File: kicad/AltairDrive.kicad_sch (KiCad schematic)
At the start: 39 parts, among them J1 Conn_02x20_Odd_Even, J2 SERIAL, J3 Conn_01x03_Pin, SW2 SW_PWR, SW3 SW_PWR

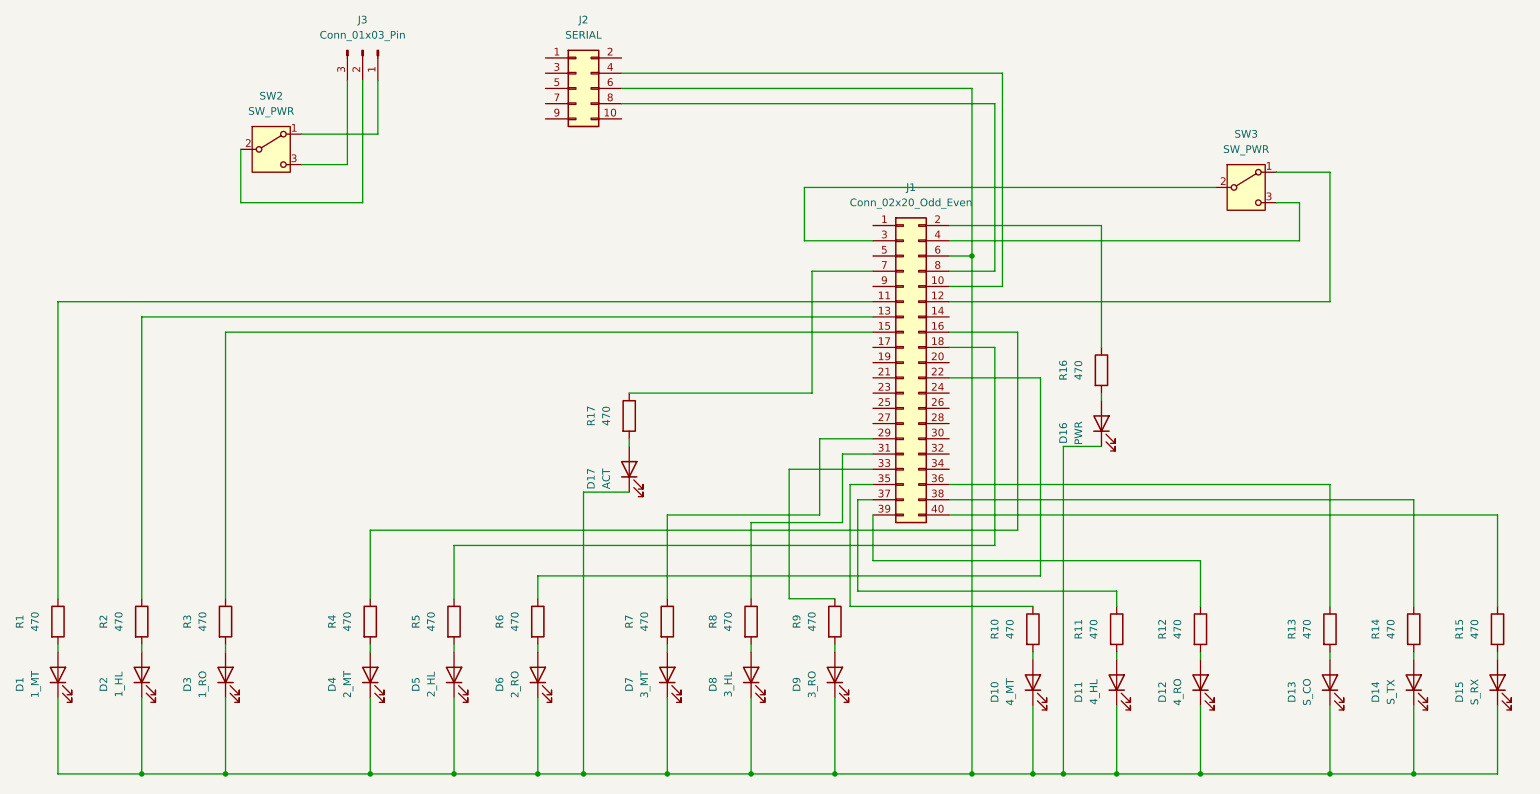
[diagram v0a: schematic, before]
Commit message: kicad files for front panel
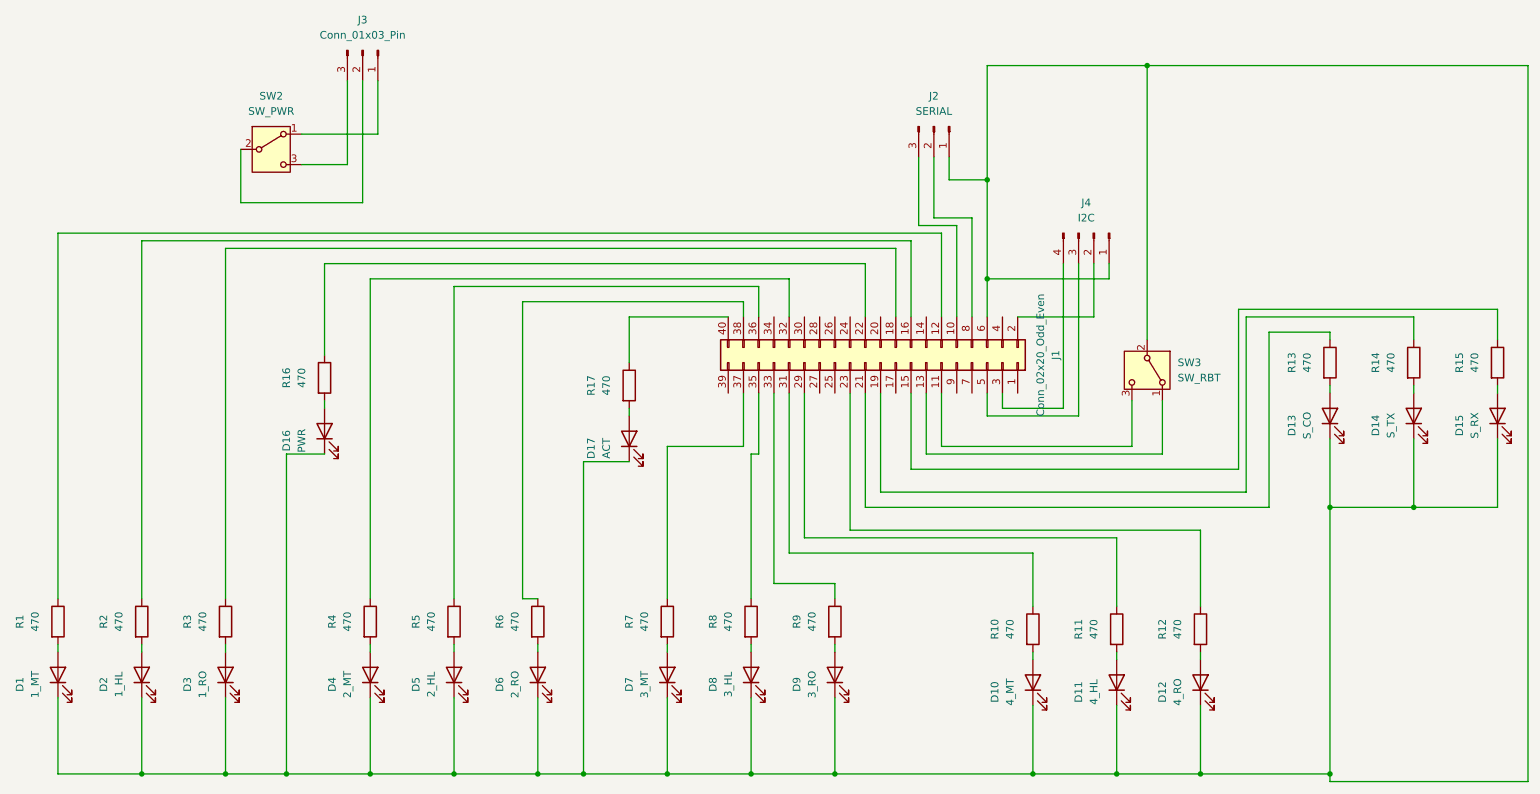
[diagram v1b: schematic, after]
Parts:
- removed J2: SERIAL, Connector_PinHeader_2.54mm:PinHeader_2x05_P2.54mm_Horizontal, symbol Connector_Generic:Conn_02x05_Odd_Even
- added J2: SERIAL, Connector:FanPinHeader_1x03_P2.54mm_Vertical, symbol Connector:Conn_01x03_Pin
- added J4: I2C, Connector:FanPinHeader_1x04_P2.54mm_Vertical, symbol Connector:Conn_01x04_Pin
- J3: footprint (none) -> Connector:FanPinHeader_1x03_P2.54mm_Vertical
- SW2: footprint (none) -> MrEppot:E-Switch
- SW3: value SW_PWR -> SW_RBT; footprint (none) -> MrEppot:E-Switch
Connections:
- net at R5.1: now also J1.36 (Pin_36); no longer J1.18 (Pin_18)
- net at R13.1: now also J1.21 (Pin_21); no longer J1.36 (Pin_36)
- net at R10.1: now also J1.31 (Pin_31); no longer J1.35 (Pin_35)
- net at D1.1 (K), D10.1 (K), D11.1 (K)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: now also SW3.2 (B), J2.1 (Pin_1), J4.1 (Pin_1)
- net at R12.1: now also J1.23 (Pin_23); no longer J1.39 (Pin_39)
- net at R14.1: now also J1.19 (Pin_19); no longer J1.38 (Pin_38)
- net at SW3.1 (A): now also J1.13 (Pin_13); no longer J1.12 (Pin_12)
- net at J1.3 (Pin_3): now also J4.4 (Pin_4); no longer SW3.2 (B)
- net at SW3.3 (C): now also J1.11 (Pin_11); no longer J1.4 (Pin_4)
- net at R11.1: now also J1.29 (Pin_29); no longer J1.37 (Pin_37)
- net at J1.10 (Pin_10): now also J2.3 (Pin_3)
- net at J1.8 (Pin_8): now also J2.2 (Pin_2)
- net at R2.1: now also J1.16 (Pin_16); no longer J1.13 (Pin_13)
- net at R8.1: now also J1.35 (Pin_35); no longer J1.31 (Pin_31)
- net at R15.1: now also J1.15 (Pin_15); no longer J1.40 (Pin_40)
- net at R1.1: now also J1.12 (Pin_12); no longer J1.11 (Pin_11)
- net at R6.1: now also J1.38 (Pin_38); no longer J1.22 (Pin_22)
- net at J1.2 (Pin_2): now also J4.2 (Pin_2); no longer R16.1
- net at R17.1: now also J1.40 (Pin_40); no longer J1.7 (Pin_7)
- net at R7.1: now also J1.37 (Pin_37); no longer J1.29 (Pin_29)
- net at R4.1: now also J1.32 (Pin_32); no longer J1.16 (Pin_16)
- net at R3.1: now also J1.18 (Pin_18); no longer J1.15 (Pin_15)
- net at J1.5 (Pin_5): now also J4.3 (Pin_3)
- new net: J1.22 (Pin_22), R16.1
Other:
- moved on the sheet: D13, D14, D15, D16, D17, J1, R13, R14, R15, R16, R17, SW3
